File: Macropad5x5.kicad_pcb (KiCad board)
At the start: 4 copper layers, 120.5 x 120.2 mm, 100 parts, among them M1 MountingHole, M2 MountingHole, M3 MountingHole, M4 MountingHole, M5 MountingHole, M6 MountingHole, M7 MountingHole, SW1 SW_Push, SW2 SW_Push, U1 PicoW, U4 SN74LV1T125DBV

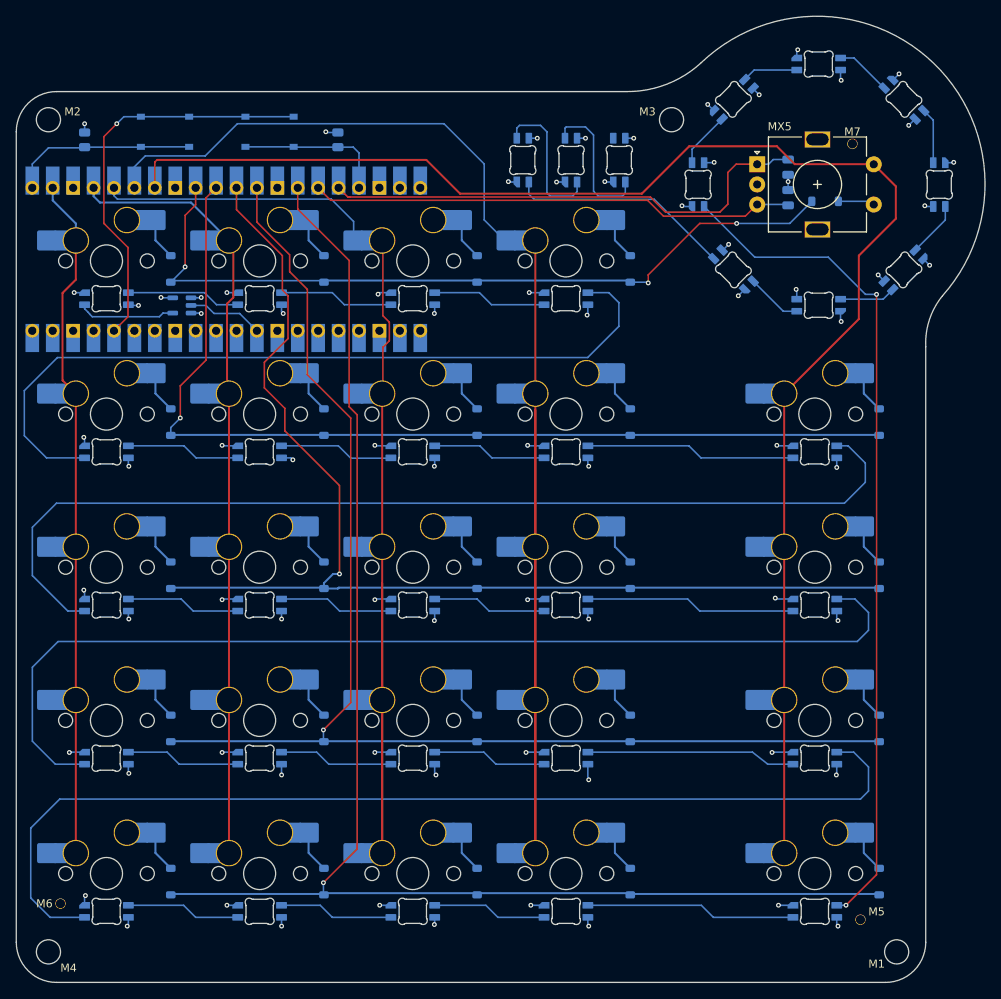
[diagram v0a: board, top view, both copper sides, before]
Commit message: Updated 3d models.
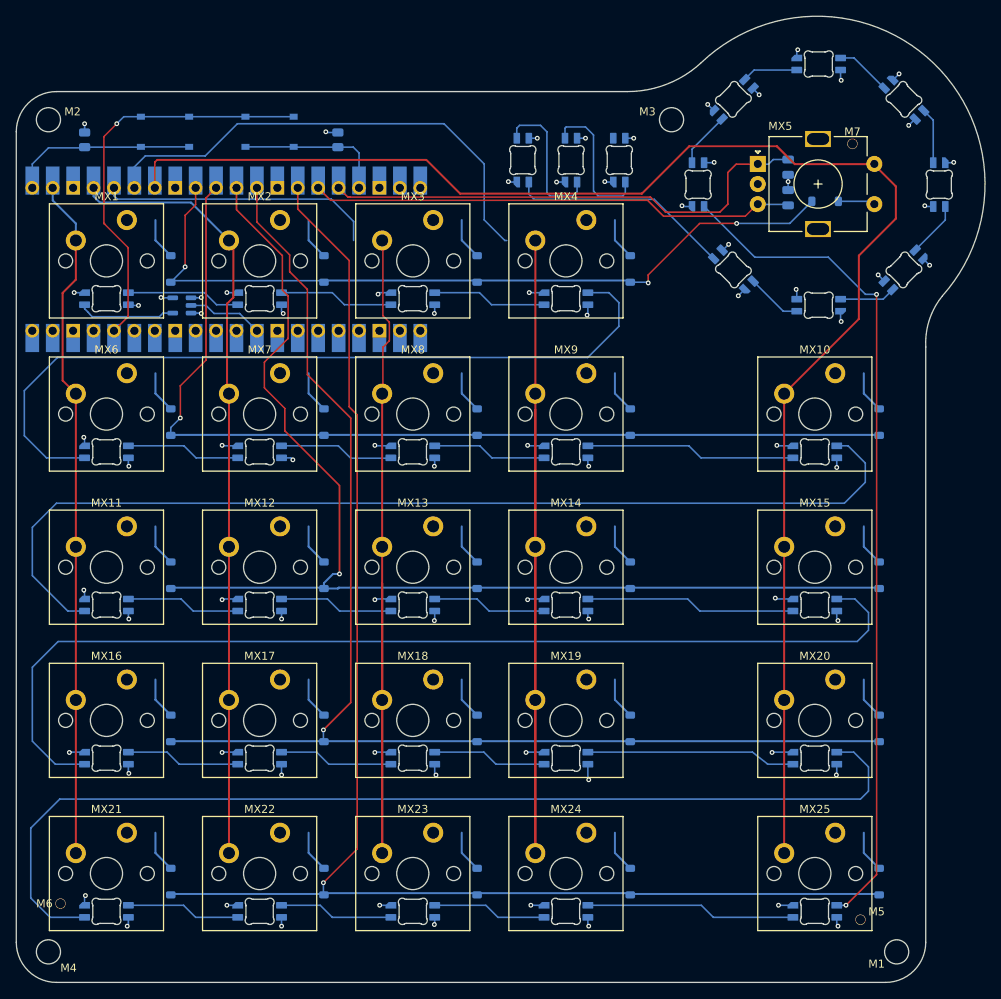
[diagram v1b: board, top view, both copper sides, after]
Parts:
- MX1, MX11, MX12, MX13, MX14, MX16, MX17, MX18, MX19, MX2, MX21, MX22, MX23, MX24, MX3, MX4, MX6, MX7, MX8, MX9: footprint PCM_marbastlib-mx:SW_MX_HS_CPG151101S11_1u -> Macropad:SW_Cherry_MX_PCB_1.00u; moved to F.Cu
- MX10, MX15, MX20, MX25: footprint PCM_marbastlib-mx:SW_MX_HS_CPG151101S11_1.25u -> Macropad:SW_Cherry_MX_PCB_1.25u; moved to F.Cu
- MX5: footprint Rotary_Encoder:RotaryEncoder_Alps_EC11E-Switch_Vertical_H20mm -> Macropad:RotaryEncoder_Alps_EC11E-Switch_Vertical_H20mm
- moved MX5 7.96 mm to (147.7, 59.5)
- turned MX1 to 0 degrees
- turned MX10 to 0 degrees
- turned MX11 to 0 degrees
- turned MX12 to 0 degrees
- turned MX13 to 0 degrees
- turned MX14 to 0 degrees
- turned MX15 to 0 degrees
- turned MX16 to 0 degrees
- turned MX17 to 0 degrees
- turned MX18 to 0 degrees
- turned MX19 to 0 degrees
- turned MX2 to 0 degrees
- turned MX20 to 0 degrees
- turned MX21 to 0 degrees
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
